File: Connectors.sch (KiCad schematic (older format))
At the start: 8 parts, among them J201 Conn_01x10, J202 Conn_ARM_JTAG_SWD_10, J203 Conn_02x03_Counter_Clockwise, J204 USB_B_Micro, J205 Conn_01x04

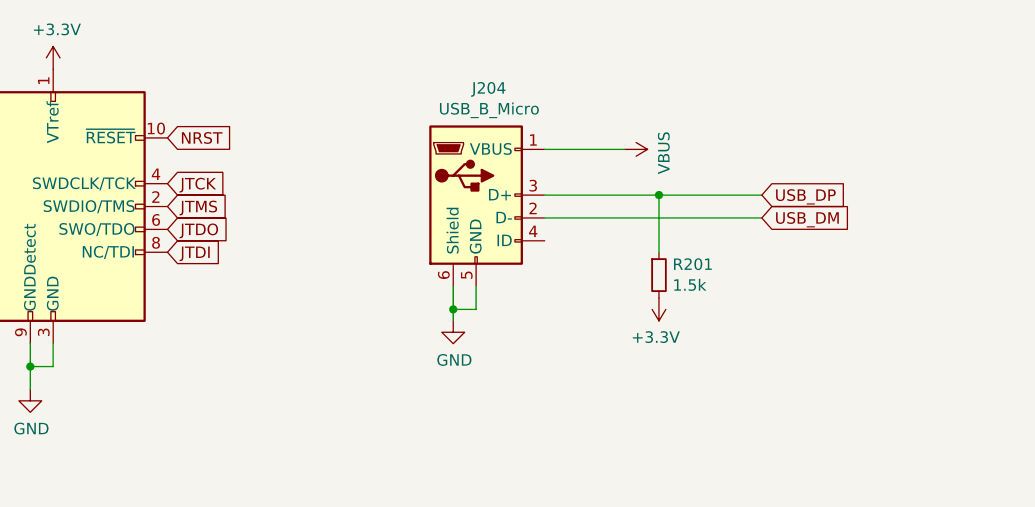
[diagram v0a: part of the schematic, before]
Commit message: more work on schematic and layout
Signed-off-by: Thomas Schmid <tom@binary-kitchen.de>
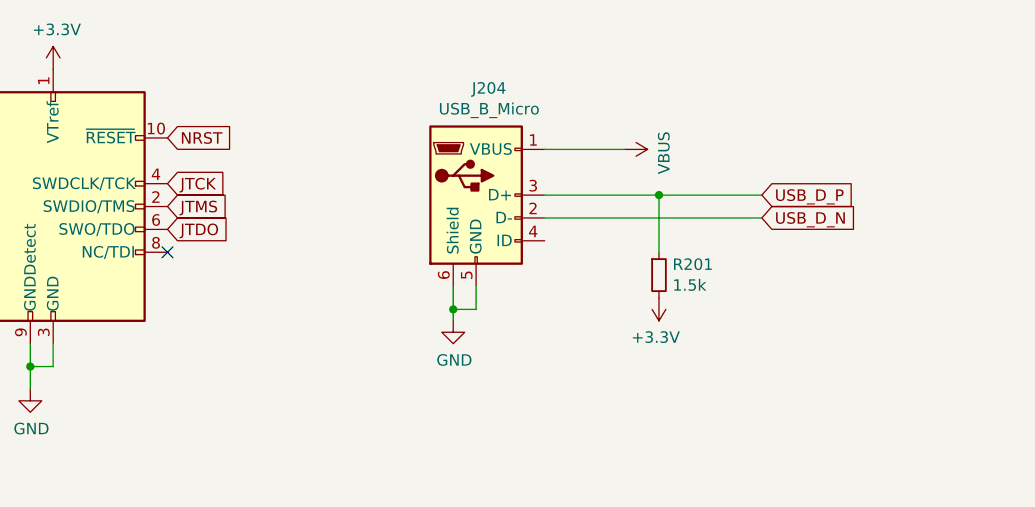
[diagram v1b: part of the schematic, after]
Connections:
- net JTDI: no longer names the net of J202.8 (NC/TDI)
- net USB_DM renamed USB_D_N
- net USB_DP renamed USB_D_P
- no-connect marks 0 -> 1
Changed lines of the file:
@@
 Wire Wire Line
 	1900 2200 1900 2100
-Text GLabel 2500 1700 2    50   Input ~ 0
-JTDI
 Text GLabel 1400 3550 0    50   Input ~ 0
 PYRO2_LOW
@@
 	4150 1550 5100 1550
 Text GLabel 5100 1450 2    50   Input ~ 0
-USB_DP
+USB_D_P
 Text GLabel 5100 1550 2    50   Input ~ 0
-USB_DM
+USB_D_N
 Text GLabel 1400 3050 0    50   Input ~ 0
 PYRO0_HIGH
@@
 	8350 1400 8350 1250
 Connection ~ 8350 1250
+NoConn ~ 2500 1700
 $EndSCHEMATC

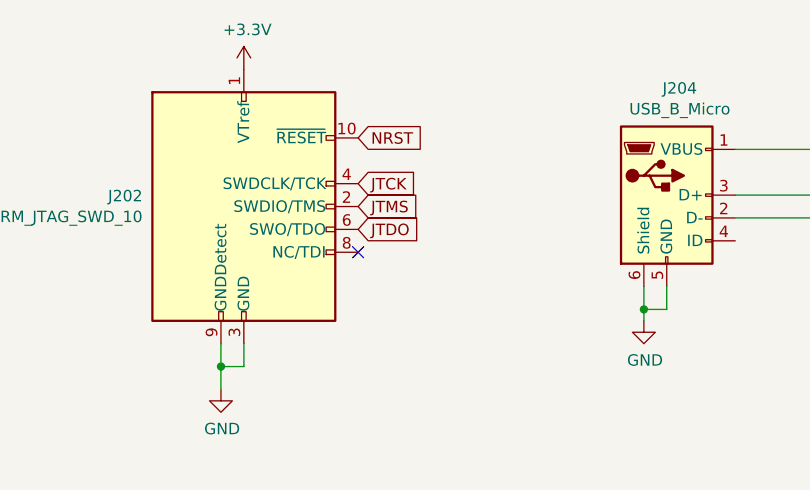
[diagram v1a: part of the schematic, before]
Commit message: major work on layout. nearly finished
Signed-off-by: Thomas Schmid <tom@binary-kitchen.de>
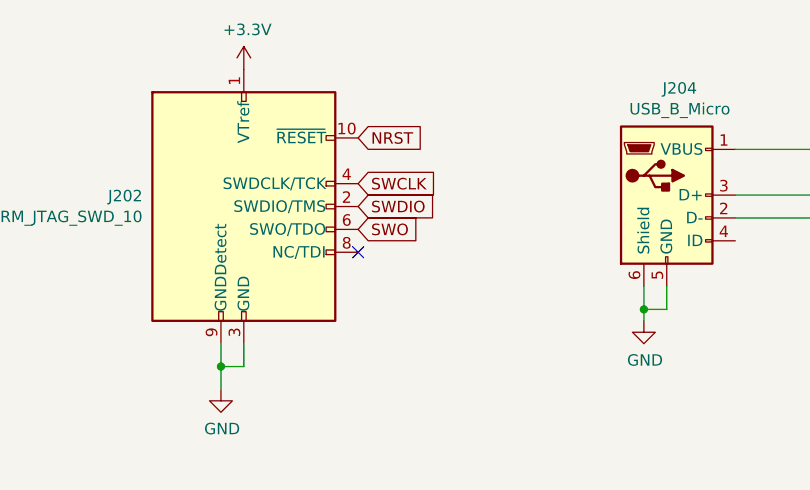
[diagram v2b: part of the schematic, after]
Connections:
- net JTCK renamed SWCLK
- net JTDO renamed SWO
- net JTMS renamed SWDIO
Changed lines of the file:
@@
 NRST
 Text GLabel 2500 1400 2    50   Input ~ 0
-JTCK
+SWCLK
 Text GLabel 2500 1500 2    50   Input ~ 0
-JTMS
+SWDIO
 Text GLabel 2500 1600 2    50   Input ~ 0
-JTDO
+SWO
 $Comp
 L power:+3.3V #PWR0204
